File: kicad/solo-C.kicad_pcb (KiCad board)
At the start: 4 copper layers, 33.5 x 15 mm, 41 parts, among them P1 USB_C_Plug, T1 TLV742p, U1 LPC55S28JEV98K

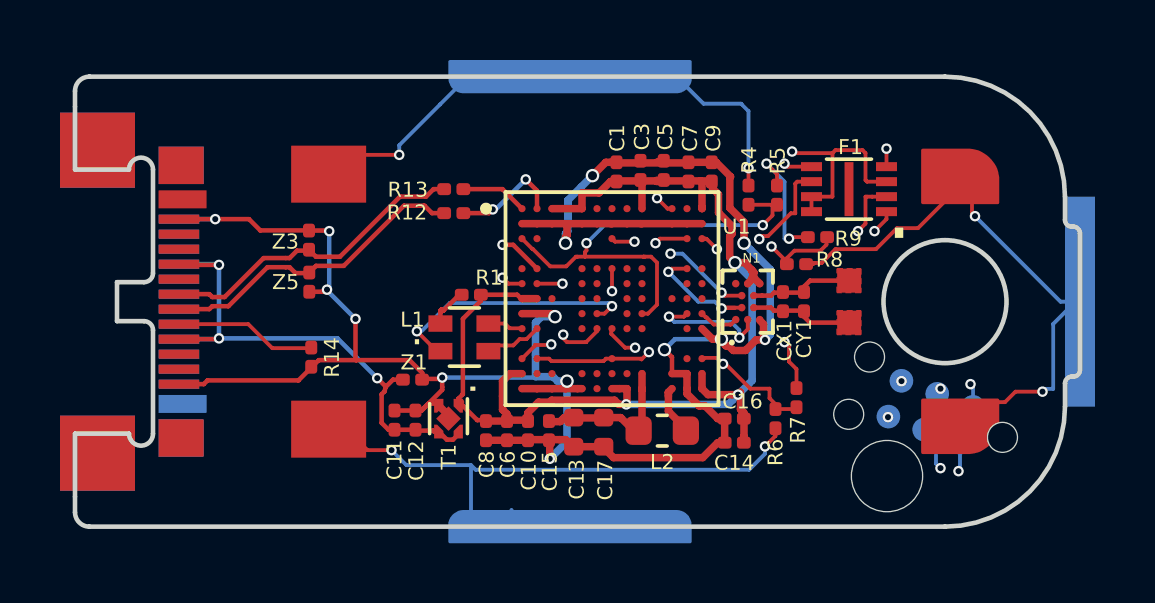
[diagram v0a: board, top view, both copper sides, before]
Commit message: new nfc chip layout
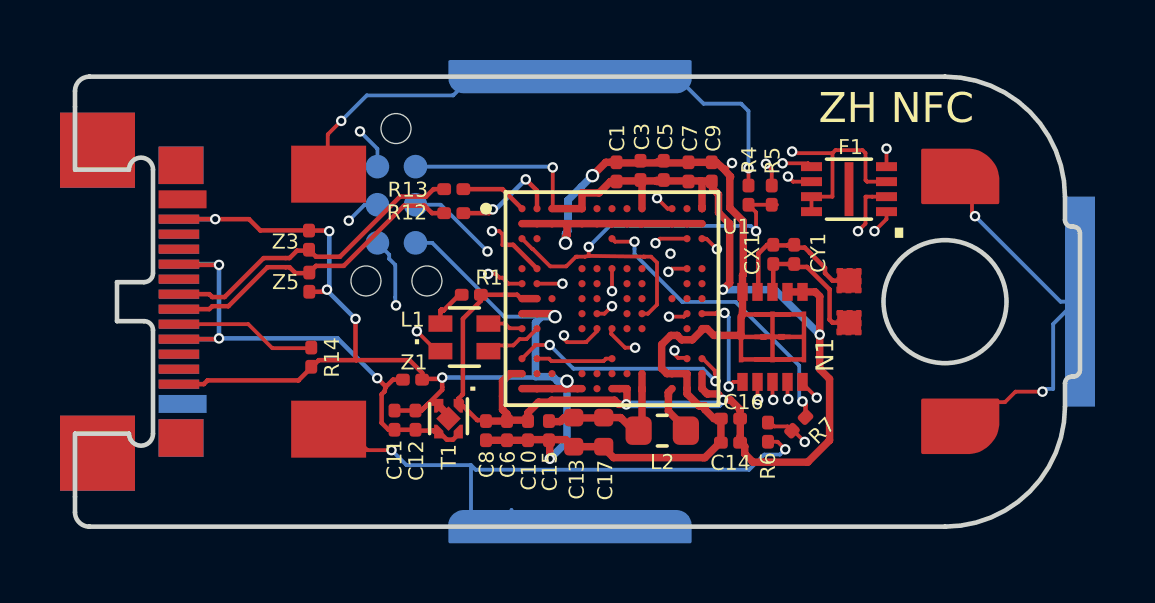
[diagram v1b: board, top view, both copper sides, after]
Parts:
- removed R8: 10k, solo:0201_R
- removed R9: 1M, solo:0201_R
- N1: value AS3953-CSP -> FM11NC08I; footprint solo:AS3953_CSP -> solo:MLPD3X3
- moved D1 20.3 mm to (127.3, 54.0), turned to 270 degrees
- moved N1 1.85 mm to (140.2, 58.2), turned to 270 degrees
- moved CY1 1.61 mm to (140.0, 56.9)
- moved CX1 1.61 mm to (139.3, 56.9)
- moved R7 0.88 mm to (140.1, 62.6), turned to 45 degrees
- moved R6 0.51 mm to (139.1, 62.9)
- moved R5 0.18 mm to (139.2, 55.0)
- moved C14 0.12 mm to (137.8, 63.2)
- moved C16 0.12 mm to (137.8, 62.4)
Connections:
- U1 pad L12: Net-(U1-PadL12) -> /solo/Sheet5DDC9C58/NFC_GPIO
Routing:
- net /solo/Sheet5DDC9C58/SWDIO: track 19.9 -> 9.42 mm
- net /solo/Sheet5DDC9C58/SENSE3: track 12.9 -> 2.62 mm, vias 2 -> 0
- net /solo/nRESET: track 18.2 -> 8.64 mm
- net /solo/Sheet5DDC9C58/SWCLK: track 17.2 -> 7.82 mm
- net /solo/Sheet5DDC9C58/NFC_GPIO: track 0.00 -> 6.89 mm, vias 0 -> 2
- net /CAP3: track 24.7 -> 18.3 mm
- net /solo/Sheet5DDC9C58/SWO: track 13.9 -> 8.99 mm
- net /solo/Sheet5DDC9C58/SPI_MISO: track 20.9 -> 25.0 mm
- net /solo/Sheet5DDC9C58/SPI_MOSI: track 10.3 -> 13.4 mm
- net +3V3: track 50.5 -> 53.5 mm, vias 4 -> 5
- net GNDREF: track 90.5 -> 87.5 mm, vias 16 -> 12
- net /solo/Sheet5DDC9C58/SENSE2: track 11.5 -> 14.3 mm, vias 2 -> 3
- net /solo/Sheet5DDC9C58/SPI_SS: track 1.34 -> 3.77 mm, vias 0 -> 2
- net /NFC+: track 3.52 -> 5.04 mm
- net /NFC-: track 3.50 -> 4.94 mm
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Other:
- board text added: "ZH NFC"
